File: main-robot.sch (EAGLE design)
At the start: 56 parts, among them CON1 AX12, CON2 AX12, CON3 GENERIC-4PIN53253, SW1 SWITCH-SPDT-H, SW2 PUSH-BUTTON436331045822, SW3 PUSH-BUTTON436331045822, SW4 PUSH-BUTTON436331045822, SW5 PUSH-BUTTON436331045822, SW6 PUSH-BUTTON436331045822, SW7 PUSH-BUTTON436331045822, U1 TEENSY_3.5_DIL+4

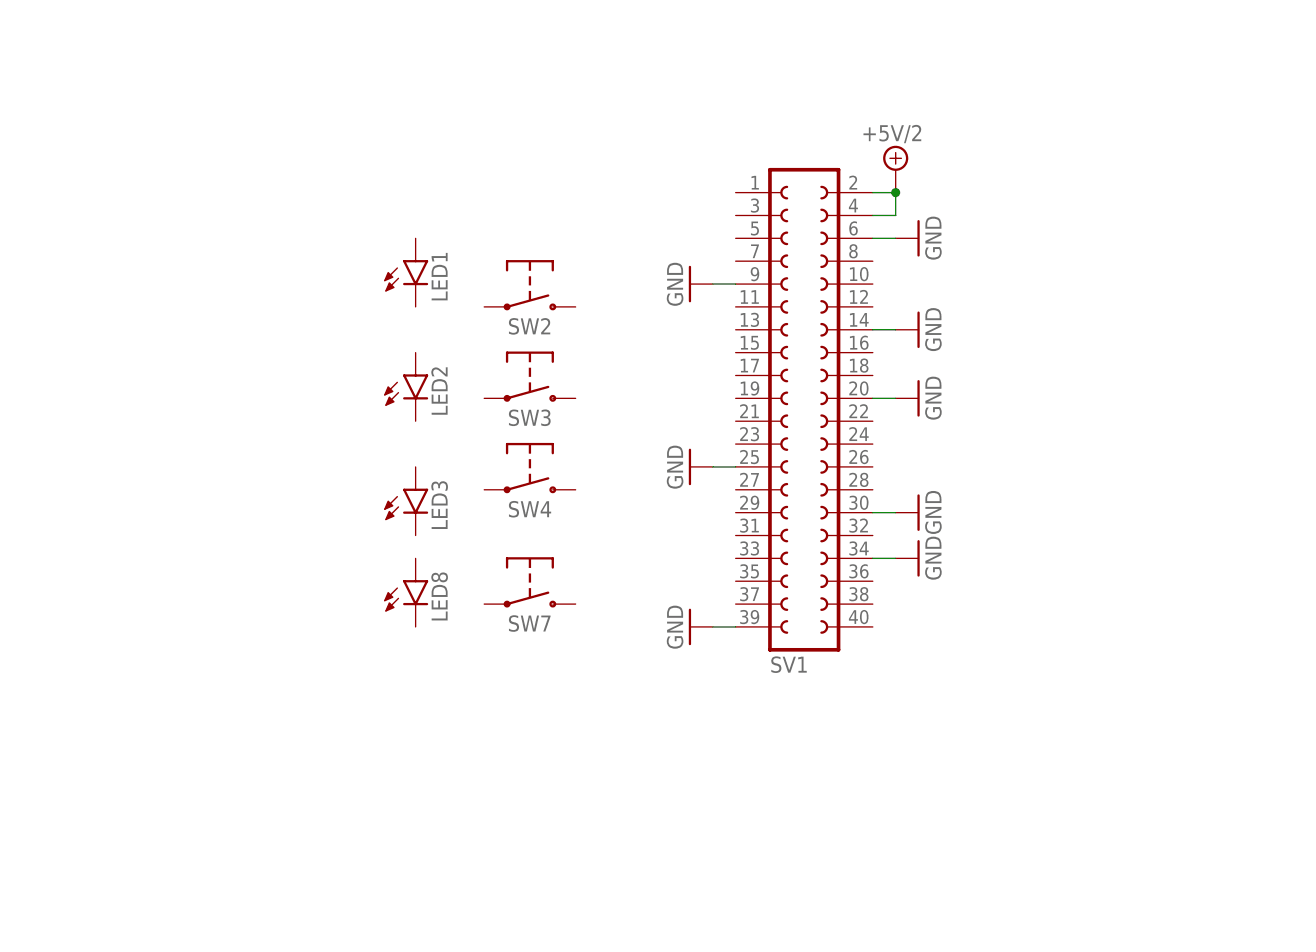
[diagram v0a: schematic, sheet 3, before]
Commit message: v1 schematics
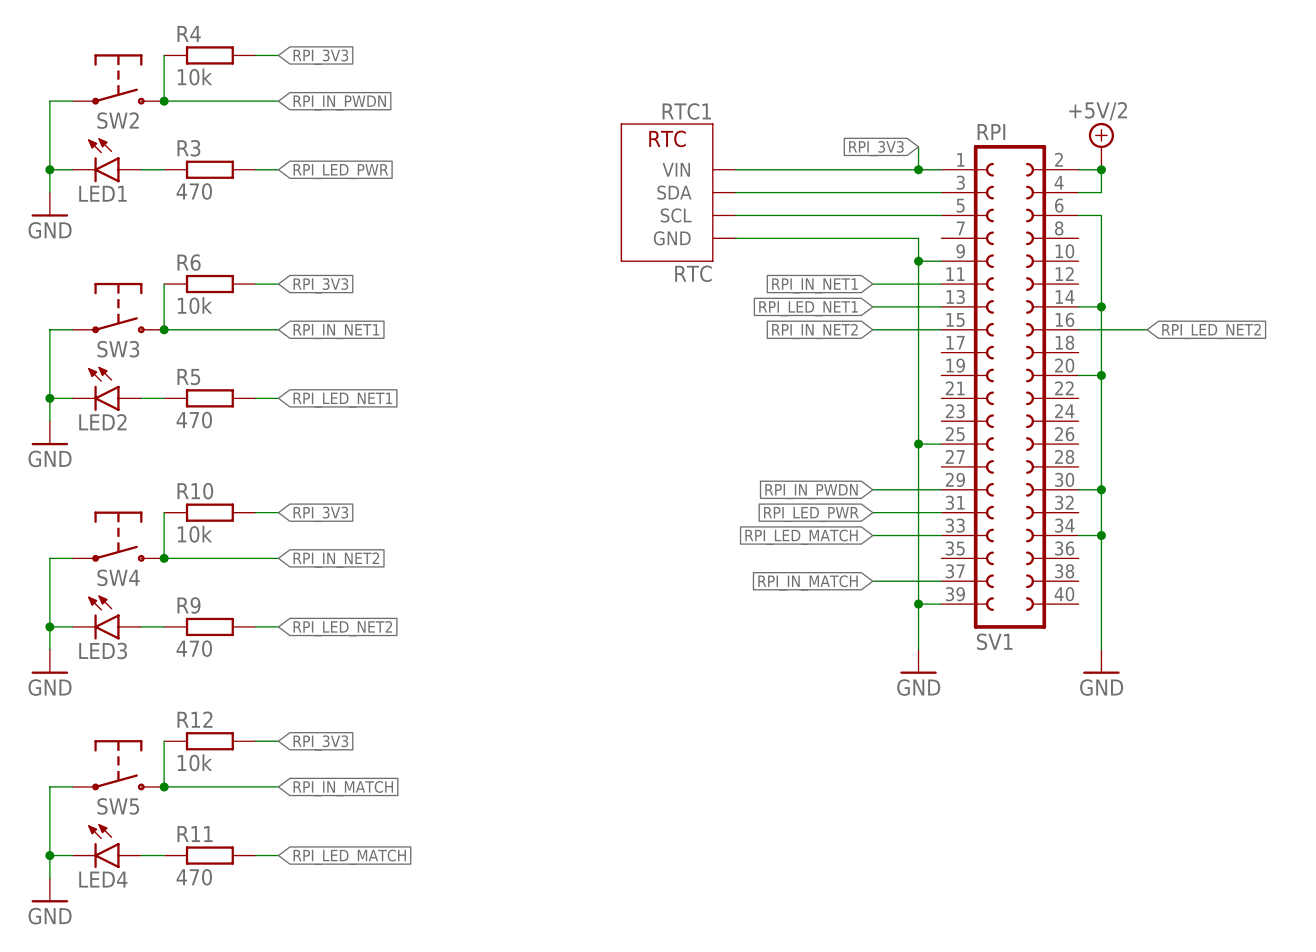
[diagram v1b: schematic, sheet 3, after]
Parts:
- added R10, R12, R14, R16, R4, R6: 10k, resistor:R-EU_R0805
- added R11, R13, R15, R17, R18, R3, R5, R9: 470, resistor:R-EU_R0805
- added RTC1: RTC, rtc-raspberry-pi:RTC
- D2: value (none) -> SS56B
- JP1: value (none) -> VUSB
- SV1: value (none) -> RPI
- SW3, SW4: value PUSH-BUTTON436331045822 -> PUSH-BUTTON; device push-button:PUSH-BUTTON436331045822 -> push-button:PUSH-BUTTON
- U1: device Teensy_libSG:TEENSY_3.5_DIL+4 -> teensy:TEENSY_3.5_DIL+4
- renumbered CON3 to FLAG
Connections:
- new net AX12_DATA_LV: U1.10/TX2/PWM, U1.9/RX2/PWM
- new net CS: R10.2, R9.1
- new net EXT_DATA_LV: U1.7/RX3/PWM, U1.8/TX3/PWM
- new net FLAG_CS: U1.16/A2
- new net FLAG_INA: U1.23/A9/PWM
- new net FLAG_INB: U1.22/A8/PWM
- new net FLAG_PWM: U1.21/A7/PWM
- new net FLAG_SEL: U1.20/A6/PWM
- new net IN_COLOR_A: R16.1, SW7.P$2, U1.25
- new net IN_COLOR_B: R14.1, SW6.P$2, U1.26
- new net IN_JUMPER: C10.2, R7.2, R8.2, U1.6/PWM
- new net LED_COLOR_A: R15.2, U1.35/A16/PWM
- new net LED_COLOR_B: R13.2, U1.36/A17/PWM
- new net LED_DATA_LV: U1.24
- new net LED_DEBUG_A: R17.2, U1.37/A18/SCL1/PWM
- new net LED_DEBUG_B: R18.2, U1.38/A19/SDA1/PWM
- new net MOT_CS: U1.17/A3/PWM
- new net MOT_INA: U1.2/PWM
- new net MOT_INB: U1.3/CAN0-TX/SCL2/PWM
- new net MOT_PWM: U1.4/CAN0-RX/SDA2/PWM
- new net MOT_SEL: U1.5/PWM
- new net N$13: R5.1, R9.2, RTC1.SDA, SV1.3
- new net N$14: RTC1.SCL, SV1.5
- new net N$16: LED2.A, R5.1
- new net N$17: LED3.A, R9.1
- new net N$18: LED4.A, R11.1
- new net N$19: LED7.A, R15.1
- new net N$20: LED5.A, R18.1
- new net N$21: LED6.A, R17.1
- new net N$9: LED1.A, R3.1, R5.2, R6.2
- new net PWM: R3.1
- new net RPI_3V3: R10.2, R12.2, R4.2, R6.2, RTC1.VIN, SV1.1
- new net RPI_IN_MATCH: R12.1, SV1.37, SW5.P$2
- new net RPI_IN_NET1: R6.1, SV1.11, SW3.P$2
- new net RPI_IN_NET2: R10.1, SV1.15, SW4.P$2
- new net RPI_IN_PWDN: R4.1, SV1.29, SW2.P$2
- new net RPI_LED_MATCH: R11.2, SV1.33
- new net RPI_LED_NET1: R5.2, SV1.13
- new net RPI_LED_NET2: R9.2, SV1.16
- new net RPI_LED_PWR: R3.2, SV1.31
- new net SCL_LV: U1.19/A5/SCL0
- new net SDA_LV: U1.18/A4/SDA0
- new net SEL: R4.1
- net 3V3: now also R14.2, R16.2
- net ENC_D_A: now also U1.11/MOSI0
- net ENC_D_B: now also U1.12/MISO0
- net ENC_G_A: now also U1.34/A15/RX5
- net ENC_G_B: now also U1.33/A14/TX5
- net ENC_MOT_A: now also U1.14/A0/PWM
- net ENC_MOT_B: now also U1.15/A1
- net FLAG_GPIO1: now also U1.31/A12/RX4
- net FLAG_GPIO2: now also U1.32/A13/TX4/SCK1
- net GND: now also LED1.C, LED2.C, LED3.C, LED4.C, LED5.C, LED6.C, LED7.C, LED8.C, R10.1, R6.1, RTC1.GND, SW2.P$1, SW3.P$1, SW4.P$1, SW5.P$1, SW6.P$1, SW7.P$1
- net JUMPER: now also JUMPER.1
- net N$10: now also LED8.A, R13.1; no longer C10.2, JUMPER.1, R7.2, R8.2
- net N$5: now also R3.2
- net N$8: now also R4.2
- net TOF_DATA: now also U1.0/RX1/MOSI1, U1.1/TX1/MISO1
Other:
- moved on the sheet: CON1, CON2, D2, DISPLAY, ENC_D, ENC_G, EXT_1, EXT_2, JP1, JUMPER, LED1, LED2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
